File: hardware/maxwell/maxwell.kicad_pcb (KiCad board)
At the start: 2 copper layers, 129.5 x 59.7 mm, 82 parts, among them J1 Canbus 1, J10 SPI2_B, J11 BACKUP, J12 UART4, J13 UART5, J14 I2C1, J15 GPIO, J2 Canbus 2, J3 Neopixel, J4 BOOT0, J5 SPI2_A, J6 Programmer, J7 Dynamo Input, J8 BOOT1, J9 Battery, Q1 BSS138, Q2 PSMN5R4-25YLD, Q3 NTR1P02T1, Q4 NTR1P02T1, Q5 NTR1P02T1, U1 MCP1501, U10 MIC39102, U2 SN65HVD233, U3 ITEAD_HC-05, U5 ESP-32S, U6 FGPMMOPA6C, U7 STM32F103RETx, U8 TLP188, U9 Buck Regulator, Y1 32.768k, Y2 8M

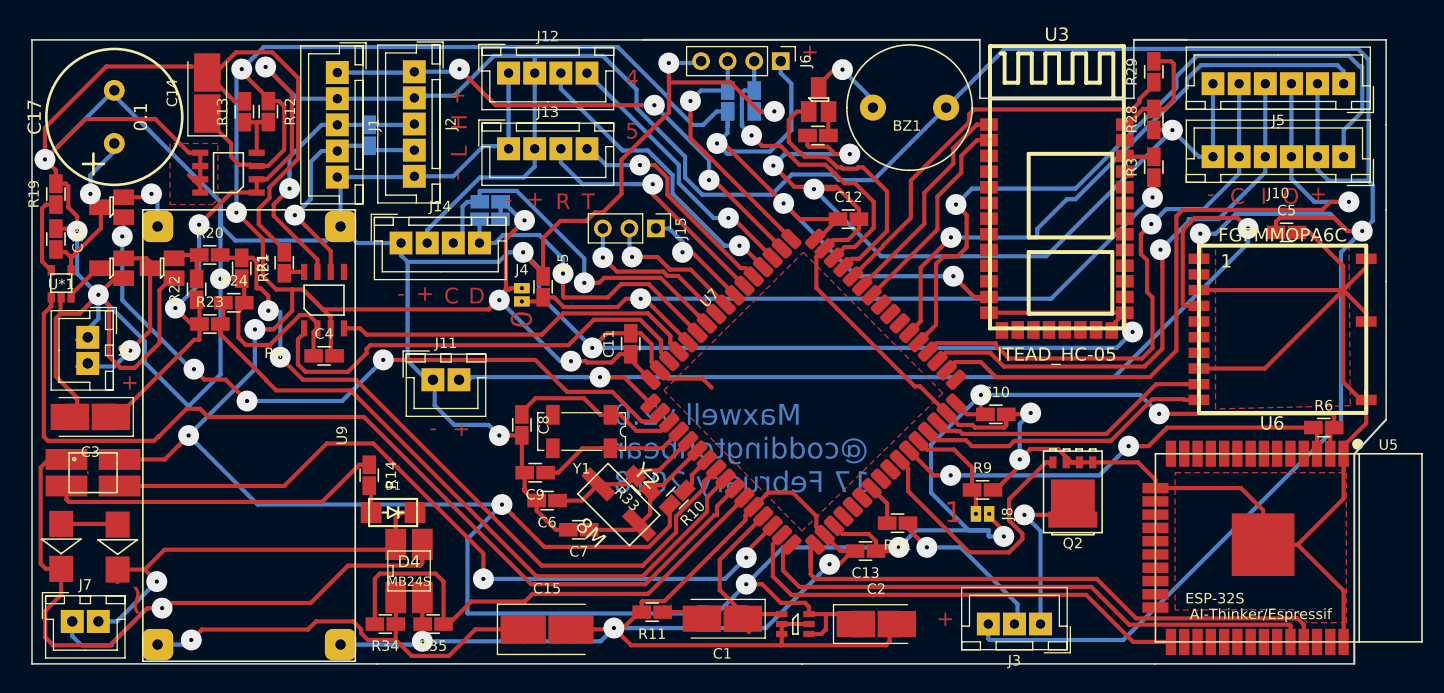
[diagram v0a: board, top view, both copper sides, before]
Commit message: Updating for manufacture.
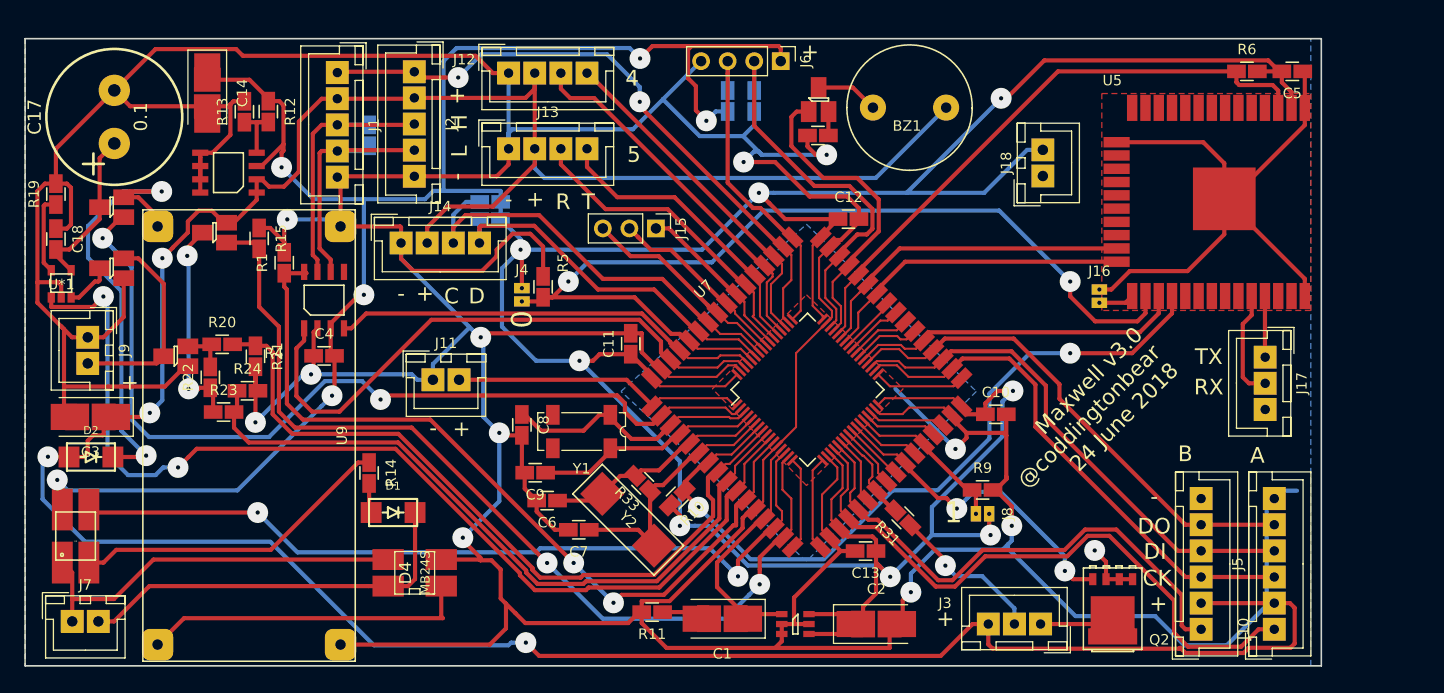
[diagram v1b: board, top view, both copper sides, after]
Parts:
- removed C15: 100u, coddingtonbear:CP_Tantalum_Case-D_EIA-7343-31_Milling
- removed D3: 18, adamgreig/agg-kicad/agg.pretty:DO-214AA-SMB
- removed R28, R35: 10k, coddingtonbear/coddingtonbear.pretty:0805_Milling
- removed R29, R3: 330, coddingtonbear/coddingtonbear.pretty:0805_Milling
- removed R34: 110k, coddingtonbear/coddingtonbear.pretty:0805_Milling
- removed U3: ITEAD_HC-05, pelrun/libKiCad/footprint/w_rf_modules.pretty:ITEAD_HC-05
- removed U6: FGPMMOPA6C, coddingtonbear/coddingtonbear.pretty:FGPMMOPA6C
- added J16: ESP_BM, coddingtonbear/coddingtonbear.pretty:Pin_Header_Straight_1x02_Pitch1.27mm_JMP, F.Cu at (175.8, 95.0)
- added J17: ESP_PROG, coddingtonbear/coddingtonbear.pretty:JST_XH_B03B-XH-A_03x2.50mm_Straight_LargePads, F.Cu at (191.6, 101.5)
- added J18: Supercap, coddingtonbear/coddingtonbear.pretty:JST_XH_B02B-XH-A_02x2.50mm_Straight_LargePads, F.Cu at (170.4, 84.1)
- added Q6: NTR1P02T1, coddingtonbear/coddingtonbear.pretty:SOT-23_LargePads, F.Cu at (91.1, 89.6)
- added R15: 10k, coddingtonbear/coddingtonbear.pretty:0805_Milling, F.Cu at (95.4, 90.1)
- D2: value 18 -> GS1M-LTP; footprint adamgreig/agg-kicad/agg.pretty:DO-214AA-SMB -> mcous/kicad-lib/footprints/diode.pretty:DO-214AC
- U7: footprint kicad-castellated-breakouts:QFP64-1.27MM-CASTELLATED -> kicad-castellated-breakouts:QFP64-1.27MM-CASTELLATED-VERS
- Y2: footprint nqbit/NQBit.pretty:HC-49USX_SMD -> cpavlina/kicad-pcblib/smd-non-ipc.pretty:Abracon-ABM2
- moved J5 52.6 mm to (192.5, 127.5), turned to 90 degrees
- moved J10 47.2 mm to (185.5, 127.5), turned to 90 degrees
- moved R6 34.9 mm to (189.9, 74.1)
- moved U5 33.3 mm to (185.9, 86.7)
- moved C5 15.4 mm to (194.2, 74.1), turned to 180 degrees
- moved Q2 11.8 mm to (177.0, 125.5)
- moved D2 9.01 mm to (79.3, 111.0), turned to 180 degrees
- moved R20 8.63 mm to (91.8, 100.2)
- moved Q5 8.52 mm to (87.4, 101.4)
- moved R21 8.52 mm to (95.0, 101.4)
- moved R22 8.52 mm to (90.7, 103.4)
- moved R23 8.52 mm to (92.0, 106.7)
- moved R24 8.52 mm to (94.3, 104.7)
- moved U8 6.28 mm to (77.8, 118.6), turned to 0 degrees
- moved Y2 1.70 mm to (130.7, 117.0), turned to 315 degrees
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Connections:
- BZ1 pad 1: +BATT -> VCC
- C3 pad 1: +BATT -> VCC
- C5 pad 1: +BATT -> GND
- C5 pad 2: GND -> +3V3
- D2 pad 1: DYNAMO_AC -> Net-(D2-Pad1)
- D2 pad 2: Net-(D2-Pad2) -> VCC
- J1 pad 2: +BATT -> VCC
- J10 pad 2: +BATT -> VCC
- J10 pad 3: SPI2_MOSI -> SPI2_SCK
- J10 pad 5: SPI2_SCK -> SPI2_MOSI
- J12 pad 2: +BATT -> VCC
- J13 pad 2: +BATT -> VCC
- J14 pad 2: +BATT -> VCC
- J2 pad 2: +BATT -> VCC
- J3 pad 3: +BATT -> VCC
- J5 pad 2: +BATT -> VCC
- J5 pad 3: SPI2_MOSI -> SPI2_SCK
- J5 pad 5: SPI2_SCK -> SPI2_MOSI
- Q3 pad 2: Net-(Q3-Pad2) -> Net-(D2-Pad1)
- R1 pad 1: Net-(R1-Pad1) -> CAN_DISABLE
- U10 pad 1: +BATT -> VCC
- U10 pad 2: +BATT -> VCC
- U2 pad 8: Net-(R1-Pad1) -> CAN_DISABLE
- U5 pad 23: Net-(U5-Pad23) -> BT_DO
- U5 pad 24: Net-(U5-Pad24) -> BT_DI
- U5 pad 26: Net-(U5-Pad26) -> BOOT0
- U5 pad 27: Net-(U5-Pad27) -> BT_KEY
- U5 pad 28: Net-(U5-Pad28) -> N_RST
- U7 pad 11: DYNAMO_VOLTAGE -> CAN_DISABLE
- U7 pad 15: ESP_BOOT_MODE -> BATT_SOURCE_DISABLE
- U7 pad 16: ESP_DI -> Net-(U7-Pad16)
- U7 pad 17: ESP_DO -> Net-(U7-Pad17)
- U7 pad 20: Net-(U7-Pad20) -> SPI2_CS_A
- U7 pad 21: Net-(U7-Pad21) -> SPI2_CS_B
- U7 pad 27: ~DISABLE_ESP -> Net-(U7-Pad27)
- U7 pad 34: SPI2_MOSI -> SPI2_SCK
- U7 pad 36: SPI2_SCK -> SPI2_MOSI
- U7 pad 37: SPI2_CS_B -> BT_KEY
- U7 pad 38: SPI2_CS_A -> Net-(U7-Pad38)
- U7 pad 44: BT_KEY -> ~DISABLE_ESP
- U9 pad 3: Net-(Q3-Pad2) -> Net-(D2-Pad1)
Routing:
- net +BATT: track 320.3 -> 20.2 mm, vias 5 -> 2
- net VCC: track 0.00 -> 291.6 mm, vias 0 -> 4
- net GND: track 845.2 -> 698.3 mm, vias 19 -> 12
- net BATT_SOURCE_DISABLE: track 0.00 -> 89.6 mm, vias 0 -> 2
- net CAN_DISABLE: track 0.00 -> 78.6 mm, vias 0 -> 2
- net +BACKUP: track 103.9 -> 28.0 mm, vias 2 -> 0
- net N_RST: track 3.80 -> 73.5 mm, vias 0 -> 2
- net ESP_DO: track 55.6 -> 5.86 mm
- net DYNAMO_VOLTAGE: track 49.5 -> 0.00 mm
- net Net-(D2-Pad1): track 0.00 -> 44.8 mm, vias 0 -> 2
- net ESP_DI: track 55.1 -> 10.5 mm
- net ESP_BOOT_MODE: track 45.0 -> 3.41 mm
- net DYNAMO_AC: track 74.1 -> 37.8 mm, vias 1 -> 0
- net SPI2_CS_B: track 72.6 -> 50.6 mm, vias 1 -> 0
- net GPS_DI: track 28.4 -> 7.08 mm
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- added copper zone on B.Cu, net GND
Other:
- board size 129.5 x 59.7 mm -> 124 x 60 mm
- board text added: "A"
- board text added: "B"
- board text added: "CK"
- board text added: "DI"
- board text added: "DO"
- board text added: "Maxwell v3.0 @coddingtonbear 24 June 2018"
- board text added: "RX"
- board text added: "TX"
- board text removed: "I"
- board text removed: "Maxwell v2.0 @coddingtonbear 17 February 2018"
- board text removed: "O"
- board text removed: "~~"
